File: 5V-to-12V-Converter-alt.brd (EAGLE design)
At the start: 14 parts, among them T1 BC337, T2 BC337

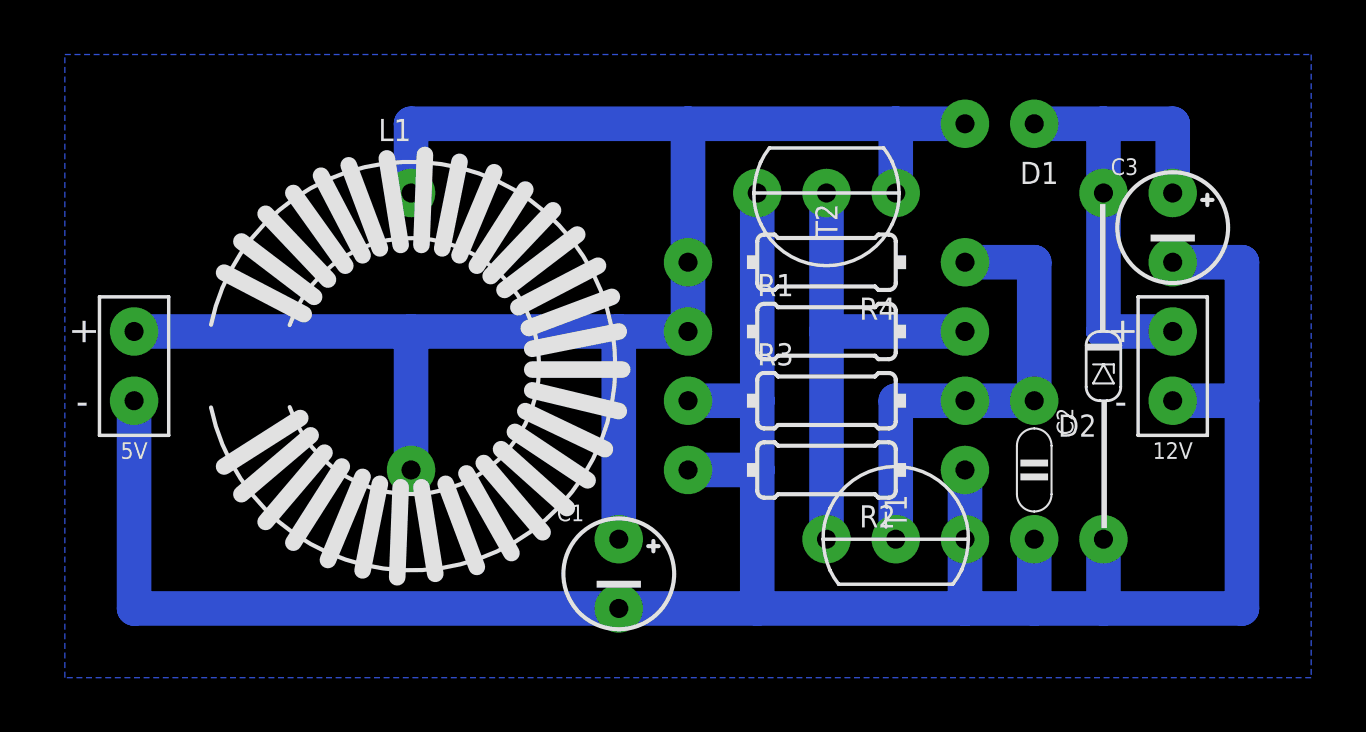
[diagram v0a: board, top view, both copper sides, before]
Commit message: ...
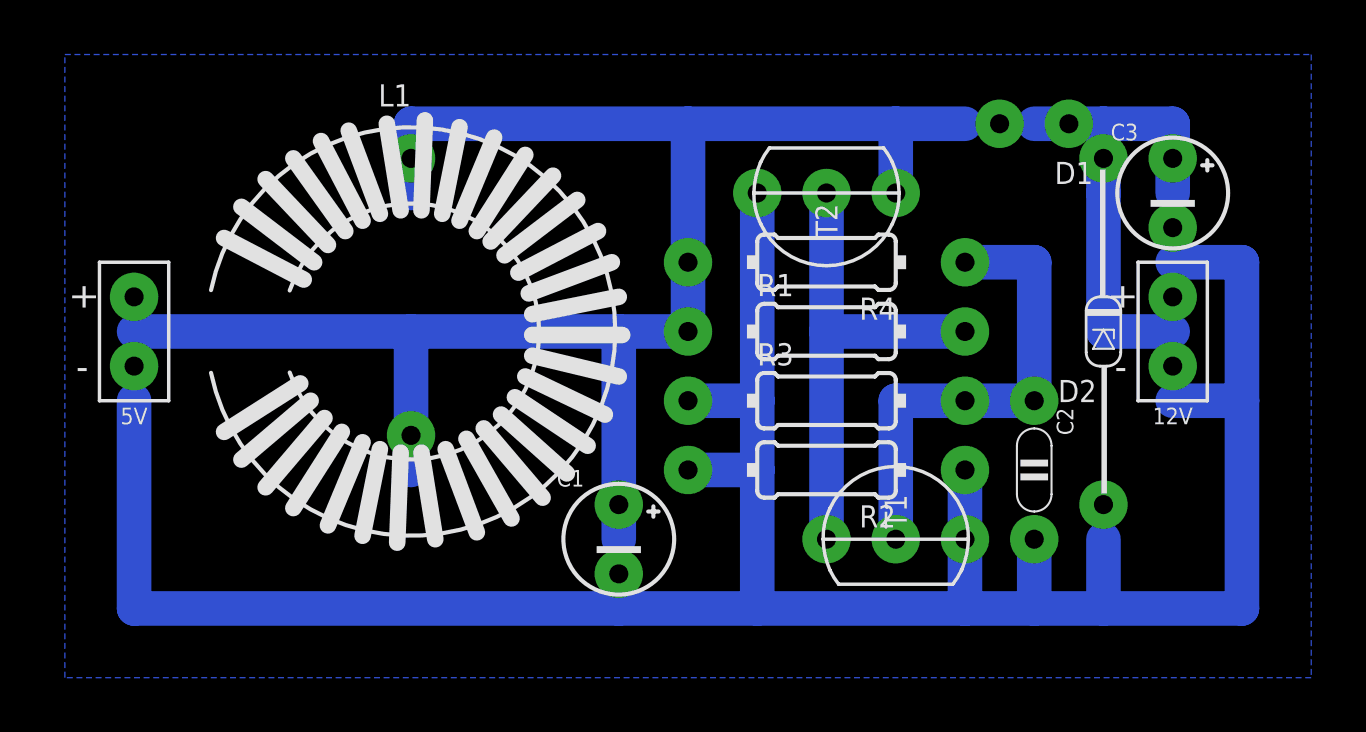
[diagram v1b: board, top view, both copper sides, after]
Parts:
- moved D1 1.27 mm to (35.6, 20.3)
- moved C1 1.27 mm to (20.3, 5.08)
- moved 12V 1.27 mm to (40.6, 12.7)
- moved 5V 1.27 mm to (2.54, 12.7)
- moved C3 1.27 mm to (40.6, 17.8)
- moved D2 1.27 mm to (38.1, 12.7)
- moved L1 1.27 mm to (12.7, 12.7)

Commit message: ...
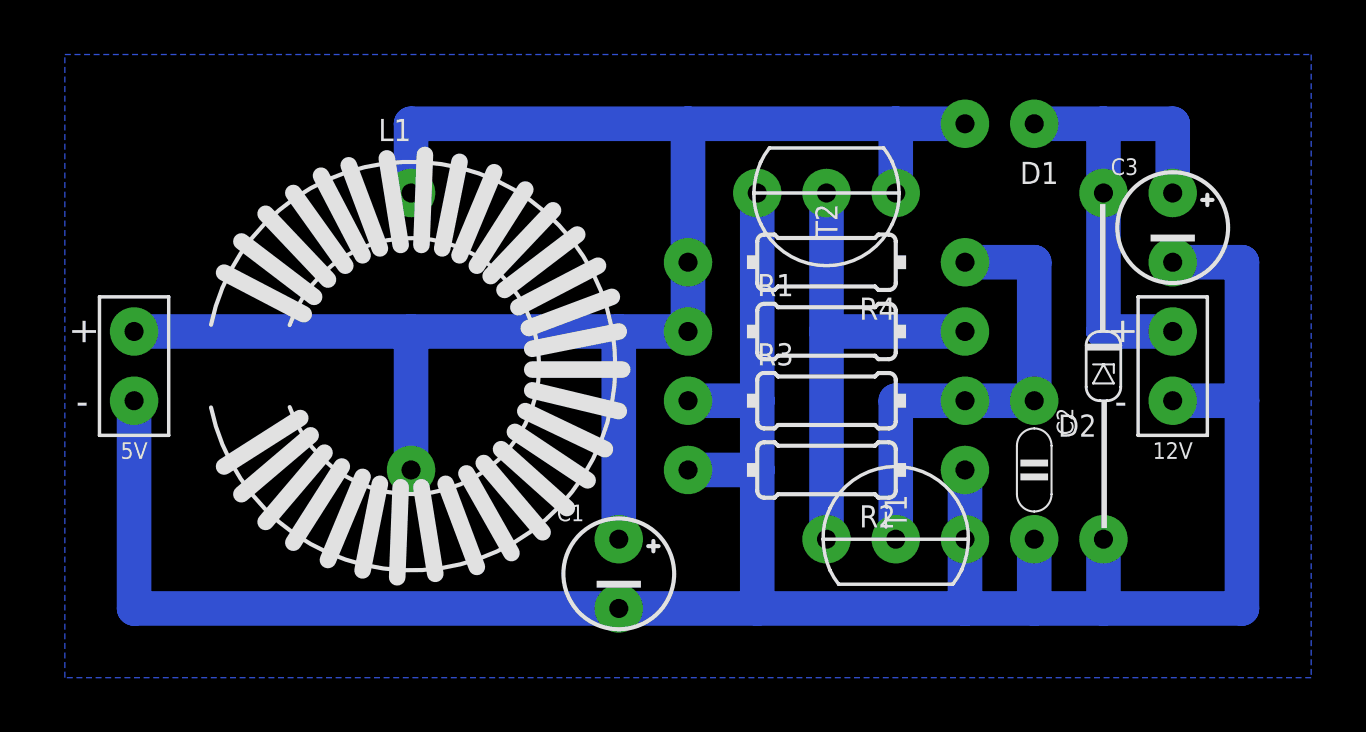
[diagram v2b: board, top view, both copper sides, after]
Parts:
- moved D1 1.27 mm to (34.3, 20.3)
- moved C1 1.27 mm to (20.3, 3.81)
- moved 12V 1.27 mm to (40.6, 11.4)
- moved 5V 1.27 mm to (2.54, 11.4)
- moved C3 1.27 mm to (40.6, 16.5)
- moved D2 1.27 mm to (38.1, 11.4)
- moved L1 1.27 mm to (12.7, 11.4)
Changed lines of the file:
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@@
       </autorouter>
       <elements>
-        <element name="C1" library="c" package="E2.5-4/V" value="47uF/16V" x="20.32" y="5.08" />
+        <element name="C1" library="c" package="E2.5-4/V" value="47uF/16V" x="20.32" y="3.81" />
         <element name="C2" library="c" package="C050-020X036" value="1nF" x="35.56" y="7.62" rot="R270" />
-        <element name="C3" library="c" package="E2.5-4/V" value="10uF/25V" x="40.64" y="17.78" />
-        <element name="D1" library="d" package="DO35-2_54A" value="1N4148" x="35.56" y="20.32" rot="R180" />
-        <element name="D2" library="d" package="DO34Z12V" value="Z=13.0V/400mW" x="38.1" y="12.7" rot="R180" />
-        <element name="L1" library="l" package="ED16-X" value="470uH/4.9 DC Ohms" x="12.7" y="12.7" />
+        <element name="C3" library="c" package="E2.5-4/V" value="10uF/25V" x="40.64" y="16.51" />
+        <element name="D1" library="d" package="DO35-2_54A" value="1N4148" x="34.29" y="20.32" rot="R180" />
+        <element name="D2" library="d" package="DO34Z12V" value="Z=13.0V/400mW" x="38.1" y="11.43" rot="R180" />
+        <element name="L1" library="l" package="ED16-X" value="470uH/4.9 DC Ohms" x="12.7" y="11.43" />
         <element name="R1" library="r" package="0204/10" value="10k" x="27.94" y="12.7" />
         <element name="R2" library="r" package="0204/10" value="6.8" x="27.94" y="7.62" rot="R180" />
@@
         <element name="T1" library="t" package="TO92-CBE" value="BC337" x="30.48" y="5.08" rot="R90" />
         <element name="T2" library="t" package="TO92-CBE" value="BC337" x="27.94" y="17.78" rot="R270" />
-        <element name="5V" library="pad" package="SPAD-+" value="" x="2.54" y="12.7" />
-        <element name="12V" library="pad" package="SPAD-+" value="" x="40.64" y="12.7" />
+        <element name="5V" library="pad" package="SPAD-+" value="" x="2.54" y="11.43" />
+        <element name="12V" library="pad" package="SPAD-+" value="" x="40.64" y="11.43" />
       </elements>
       <signals>
